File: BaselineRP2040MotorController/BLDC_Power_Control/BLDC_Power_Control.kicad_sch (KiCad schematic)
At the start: 7 parts, among them J3 3 Pin XT30 / XT60

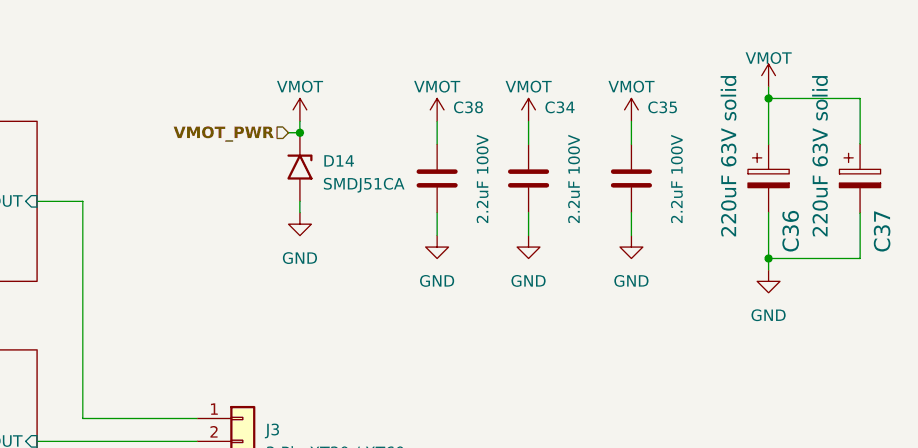
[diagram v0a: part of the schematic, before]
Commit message: Post Feedback Changes.
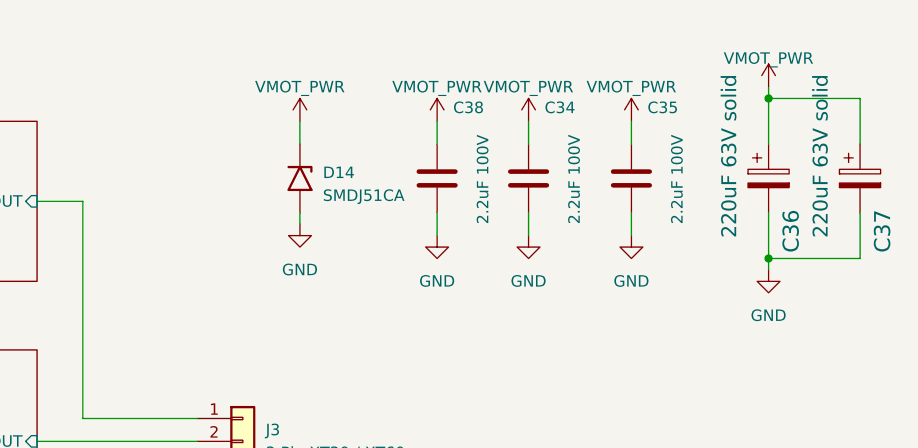
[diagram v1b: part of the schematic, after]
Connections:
- net Motor Phase ${PhaseDesignator}/${PhaseDesignator}_OUT is gone; now on net Motor Phase ${PhaseDesignator}/${PhaseDesignator}_OUT: J3.3 (Pin_3)
- net Motor Phase ${PhaseDesignator}/${PhaseDesignator}_OUT: no longer J3.1 (Pin_1)
- net VMOT renamed VMOT_PWR
- new net Motor Phase ${PhaseDesignator}/${PhaseDesignator}_OUT: J3.1 (Pin_1)
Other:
- moved on the sheet: D14
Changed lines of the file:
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@@
-	)
-	(junction
-		(at 125.73 25.4)
-		(diameter 0)
-		(color 0 0 0 0)
 	)
 	(junction
@@
 	(wire
 		(pts
-			(xy 125.73 34.29) (xy 125.73 33.02)
-		)
-		(stroke
-			(width 0)
-			(type default)
-		)
-	)
-	(wire
-		(pts
-			(xy 125.73 24.13) (xy 125.73 25.4)
+			(xy 125.73 35.56) (xy 125.73 34.29)
+		)
+		(stroke
+			(width 0)
+			(type default)
+		)
+	)
+	(wire
+		(pts
+			(xy 125.73 24.13) (xy 125.73 26.67)
 		)
 		(stroke
@@
 		(pts
 			(xy 162.56 34.29) (xy 162.56 36.83)
-		)
-		(stroke
-			(width 0)
-			(type default)
-		)
-	)
-	(wire
-		(pts
-			(xy 124.46 25.4) (xy 125.73 25.4)
 		)
 		(stroke
@@
 		(shape output)
 		(at 45.72 91.44 180)
-		(fields_autoplaced yes)
-		(effects
-			(font
-				(size 1.27 1.27)
-				(bold yes)
-			)
-			(justify right)
-		)
-	)
-	(hierarchical_label "VMOT_PWR"
-		(shape input)
-		(at 124.46 25.4 180)
 		(fields_autoplaced yes)
 		(effects
@@
 		(on_board yes)
 		(dnp no)
-		(property "Reference" "#PWR074"
+		(property "Reference" "#PWR06"
 			(at 125.73 27.94 0)
 			(effects
@@
 			)
 		)
-		(property "Value" "VMOT"
+		(property "Value" "VMOT_PWR"
 			(at 125.73 20.32 0)
 			(effects
@@
 			(project "BaselineRP2040MotorController"
 				(path "/085e5f08-c826-4caa-b8e2-0a741609456e/adfc6ecc-6038-43a2-a2be-baacb83b86f1"
-					(reference "#PWR074")
+					(reference "#PWR06")
 					(unit 1)
 				)
@@
 	(symbol
 		(lib_id "power:GND")
-		(at 125.73 34.29 0)
+		(at 125.73 35.56 0)
 		(unit 1)
 		(exclude_from_sim no)
@@
 		(fields_autoplaced yes)
 		(property "Reference" "#PWR075"
+			(at 125.73 41.91 0)
+			(effects
+				(font
+					(size 1.27 1.27)
+				)
+				(hide yes)
+			)
+		)
+		(property "Value" "GND"
 			(at 125.73 40.64 0)
 			(effects
@@
 					(size 1.27 1.27)
 				)
-				(hide yes)
-			)
-		)
-		(property "Value" "GND"
-			(at 125.73 39.37 0)
-			(effects
-				(font
-					(size 1.27 1.27)
-				)
 			)
 		)
 		(property "Footprint" ""
-			(at 125.73 34.29 0)
+			(at 125.73 35.56 0)
 			(effects
 				(font
@@
 		)
 		(property "Datasheet" ""
-			(at 125.73 34.29 0)
+			(at 125.73 35.56 0)
 			(effects
 				(font
@@
 		)
 		(property "Description" "Power symbol creates a global label with name \"GND\" , ground"
-			(at 125.73 34.29 0)
+			(at 125.73 35.56 0)
 			(effects
 				(font
@@
 	(symbol
 		(lib_id "Diode:SMF54A")
-		(at 125.73 29.21 270)
+		(at 125.73 30.48 270)
 		(unit 1)
 		(exclude_from_sim no)
@@
 		(fields_autoplaced yes)
 		(property "Reference" "D14"
-			(at 128.27 28.575 90)
+			(at 128.27 29.845 90)
 			(effects
 				(font
@@
 		)
 		(property "Value" "SMDJ51CA"
-			(at 128.27 31.115 90)
+			(at 128.27 32.385 90)
 			(effects
 				(font
@@
 		)
 		(property "Footprint" "Diode_SMD:D_SMF"
-			(at 120.65 29.21 0)
+			(at 120.65 30.48 0)
 			(effects
 				(font
@@
 		)
 		(property "Datasheet" "https://www.vishay.com/doc?85881"
-			(at 125.73 27.94 0)
+			(at 125.73 29.21 0)
 			(effects
 				(font
@@
 		)
 		(property "Description" "200W unidirectional Transil Transient Voltage Suppressor, 54Vrwm, SMF"
-			(at 125.73 29.21 0)
+			(at 125.73 30.48 0)
 			(effects
 				(font
@@
 		)
 		(property "LCSC" "C406702"
-			(at 125.73 29.21 90)
+			(at 125.73 30.48 90)
 			(effects
 				(font
@@
 			)
 		)
-		(property "Value" "VMOT"
+		(property "Value" "VMOT_PWR"
 			(at 140.97 20.32 0)
 			(effects
@@
 			)
 		)
-		(property "Value" "VMOT"
+		(property "Value" "VMOT_PWR"
 			(at 162.56 20.32 0)
 			(effects
@@
 			)
 		)
-		(property "Value" "VMOT"
+		(property "Value" "VMOT_PWR"
 			(at 151.13 20.32 0)
 			(effects
@@
 			)
 		)
-		(property "Value" "VMOT"
+		(property "Value" "VMOT_PWR"
 			(at 177.8 17.145 0)
 			(effects
